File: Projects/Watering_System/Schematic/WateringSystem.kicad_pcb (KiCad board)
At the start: 2 copper layers, 1 part

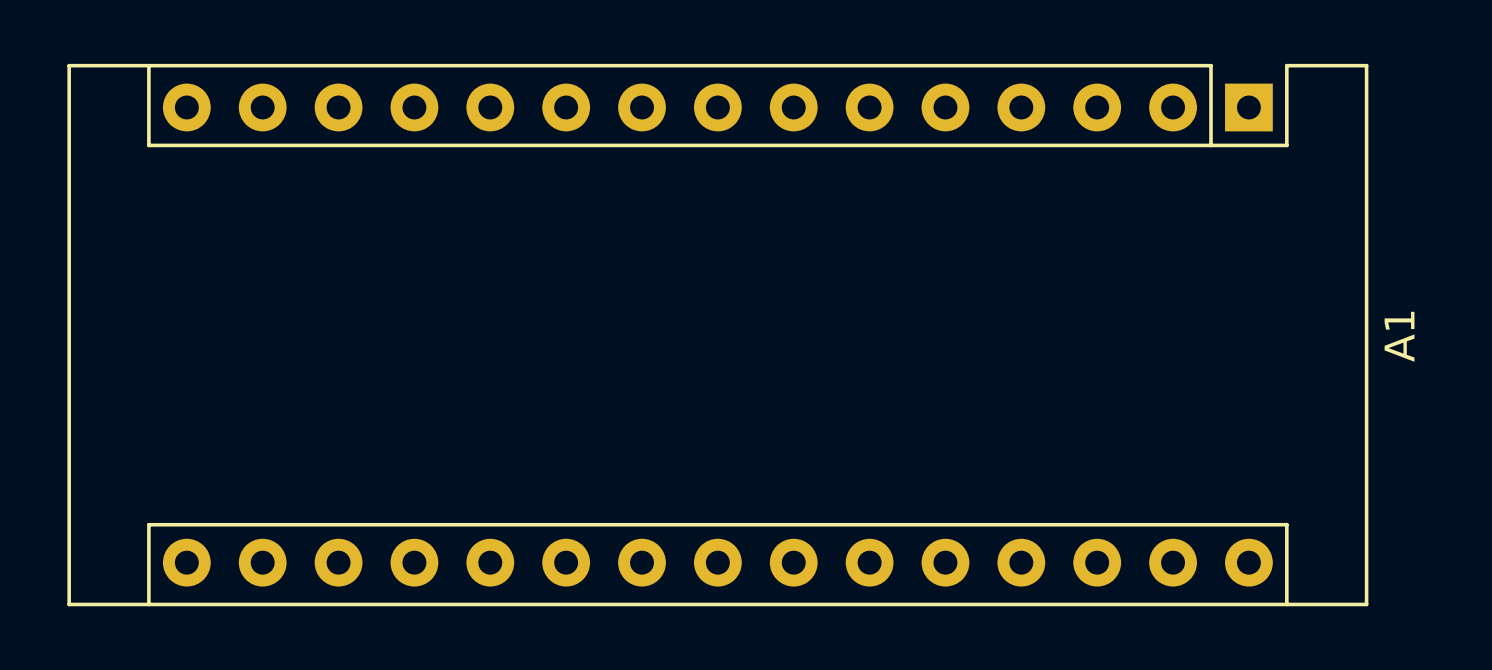
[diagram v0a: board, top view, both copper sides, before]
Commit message: add gerber files for watering project
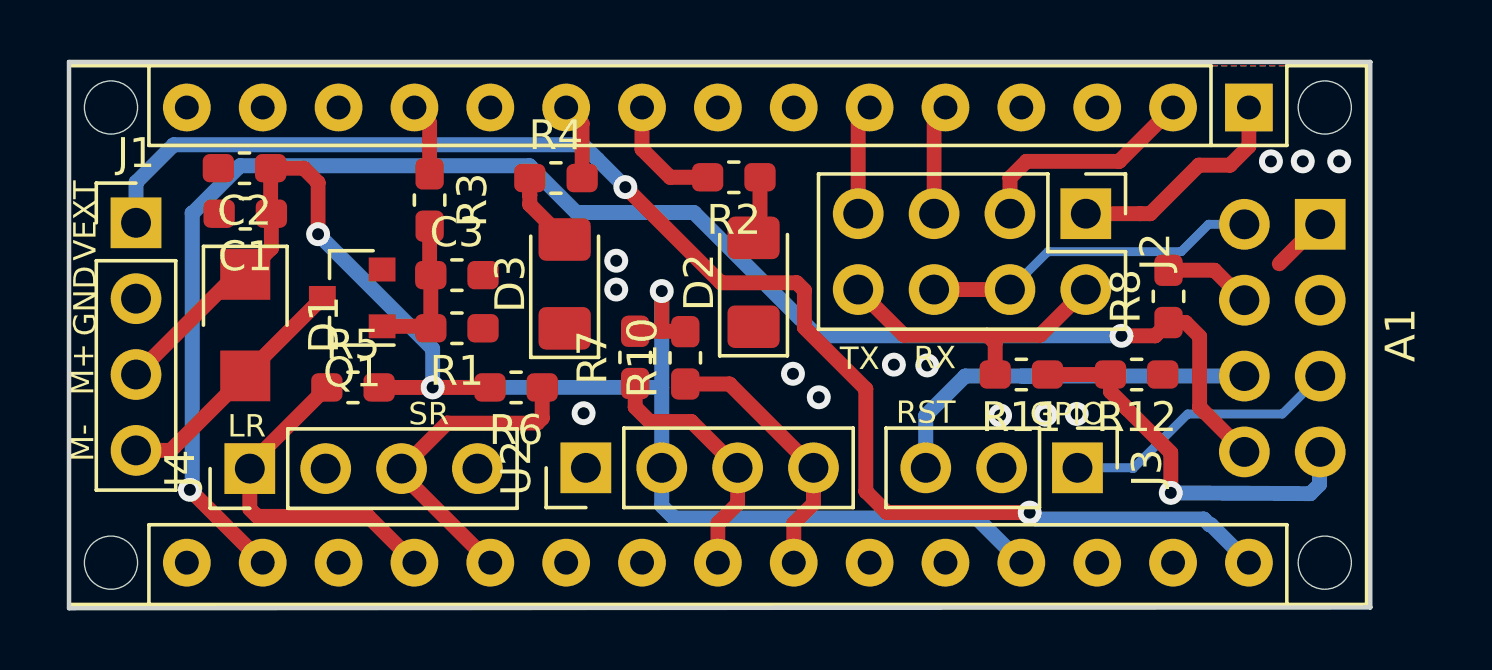
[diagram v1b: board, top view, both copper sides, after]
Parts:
- added C1: 22u, Capacitor_SMD:C_0603_1608Metric_Pad1.05x0.95mm_HandSolder, F.Cu at (69.6, 80.3)
- added C2: 1n, Capacitor_SMD:C_0603_1608Metric_Pad1.05x0.95mm_HandSolder, F.Cu at (69.5, 78.8)
- added C3: 100n, Capacitor_SMD:C_0603_1608Metric_Pad1.05x0.95mm_HandSolder, F.Cu at (76.7, 82.4)
- added D1: SS14, custom-footprints:SMA_DO-214AC, F.Cu at (69.6, 84.0)
- added D2: YELLOW, LED_SMD:LED_1206_3216Metric_Pad1.42x1.75mm_HandSolder, F.Cu at (86.6, 82.6)
- added D3: RED, LED_SMD:LED_1206_3216Metric_Pad1.42x1.75mm_HandSolder, F.Cu at (80.3, 82.7)
- added J1: MOTOR_INTERFACE, Connector_PinHeader_2.54mm:PinHeader_1x04_P2.54mm_Vertical, F.Cu at (65.9, 80.6)
- added J2: Conn_02x04_Odd_Even, Connector_PinHeader_2.54mm:PinHeader_2x04_P2.54mm_Vertical, F.Cu at (97.7, 80.3)
- added J3: FLASH_WIFI, Connector_PinHeader_2.54mm:PinHeader_1x03_P2.54mm_Vertical, F.Cu at (97.4, 88.8)
- added J4: WATER_SENSOR, Connector_PinHeader_2.54mm:PinHeader_1x04_P2.54mm_Vertical, F.Cu at (69.7, 88.8)
- added Q1: AO3400A, Package_TO_SOT_SMD:SOT-23, F.Cu at (73.2, 83.1)
- added R1: 47k, Resistor_SMD:R_0603_1608Metric_Pad1.05x0.95mm_HandSolder, F.Cu at (76.7, 84.2)
- added R10: 4k7, Resistor_SMD:R_0603_1608Metric_Pad1.05x0.95mm_HandSolder, F.Cu at (84.3, 85.1)
- added R11: 10k, Resistor_SMD:R_0603_1608Metric_Pad1.05x0.95mm_HandSolder, F.Cu at (95.6, 85.7)
- added R12: 20k, Resistor_SMD:R_0603_1608Metric_Pad1.05x0.95mm_HandSolder, F.Cu at (99.4, 85.7)
- added R2: 560, Resistor_SMD:R_0603_1608Metric_Pad1.05x0.95mm_HandSolder, F.Cu at (85.9, 79.1)
- added R3: 100, Resistor_SMD:R_0603_1608Metric_Pad1.05x0.95mm_HandSolder, F.Cu at (75.7, 79.9)
- added R4: 560, Resistor_SMD:R_0603_1608Metric_Pad1.05x0.95mm_HandSolder, F.Cu at (80.0, 79.1)
- added R5: ??, Resistor_SMD:R_0603_1608Metric_Pad1.05x0.95mm_HandSolder, F.Cu at (73.2, 86.1)
- added R6: ??, Resistor_SMD:R_0603_1608Metric_Pad1.05x0.95mm_HandSolder, F.Cu at (78.6, 86.1)
- added R7: 4k7, Resistor_SMD:R_0603_1608Metric_Pad1.05x0.95mm_HandSolder, F.Cu at (82.6, 85.1)
- added R8: 10k, Resistor_SMD:R_0603_1608Metric_Pad1.05x0.95mm_HandSolder, F.Cu at (100.5, 83.1)
- added U1: ESP8266, Connector_PinHeader_2.54mm:PinHeader_2x04_P2.54mm_Vertical, B.Cu at (105.6, 80.7)
- added U2: LCD_2x16_w_i2c, Connector_PinHeader_2.54mm:PinHeader_1x04_P2.54mm_Vertical, F.Cu at (81.0, 88.8)
- A1: footprint Module:Arduino_Nano -> Module:Arduino_Nano_WithMountingHoles
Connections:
- A1 pad 1: (no net) -> /H_TX
- A1 pad 10: (no net) -> /RED_LED
- A1 pad 12: (no net) -> Net-(A1-Pad12)
- A1 pad 17: (no net) -> /3V3
- A1 pad 19: (no net) -> /LR_LEVEL
- A1 pad 2: (no net) -> /H_RX
- A1 pad 20: (no net) -> /SR_LEVEL
- A1 pad 23: (no net) -> /SDA
- A1 pad 24: (no net) -> /SCL
- A1 pad 27: (no net) -> /5V0
- A1 pad 29: (no net) -> GND
- A1 pad 30: (no net) -> /VIN
- A1 pad 4: (no net) -> GND
- A1 pad 5: (no net) -> /S_RX
- A1 pad 6: (no net) -> /S_TX
- A1 pad 9: (no net) -> /YELLOW_LED
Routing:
- net /3V3: track 0.00 -> 54.4 mm, vias 0 -> 2
- net /5V0: track 0.00 -> 53.6 mm, vias 0 -> 3
- net /VIN: track 0.00 -> 47.7 mm, vias 0 -> 2
- net /RST_WIFI: track 0.00 -> 14.2 mm
- net Net-(R11-Pad1): track 0.00 -> 13.1 mm, vias 0 -> 1
- net /LR_LEVEL: track 0.00 -> 11.4 mm
- net /RX: track 0.00 -> 11.3 mm
- net /SR_LEVEL: track 0.00 -> 10.8 mm
- net /TX: track 0.00 -> 10.3 mm
- net /GPIO0_WIFI: track 0.00 -> 9.42 mm
- net /SCL: track 0.00 -> 8.90 mm
- net /SDA: track 0.00 -> 8.51 mm
- net /MOTOR_GND: track 0.00 -> 8.37 mm
- net /H_TX: track 0.00 -> 7.70 mm
- net /H_RX: track 0.00 -> 7.64 mm
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- added copper zone on B.Cu, net GND
- added copper zone on F.Cu, net GND
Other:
- board outline added: 43.6 x 18.3 mm
- board text added: "GND"
- board text added: "GPIO"
- board text added: "LR"
- board text added: "M+"
- board text added: "M-"
- board text added: "RST"
- board text added: "RX"
- board text added: "SR"
- board text added: "TX"
- board text added: "VEXT"
